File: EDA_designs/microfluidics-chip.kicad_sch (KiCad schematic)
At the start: 38 parts, among them J1 Conn_01x06_Pin, J10 39-53-2045, J11 Conn_01x14_Pin, J12 Conn_01x14_Pin, J13 39-53-2045, J14 39-53-2045, J15 Conn_ARM_SWD_TagConnect_TC2030, J16 Conn_01x02_Socket, J18 EJ508A, J2 Conn_01x06_Pin, J3 Conn_01x06_Pin, J4 Conn_01x06_Pin, J5 Conn_01x04_Socket, J8 39-53-2045, Q1 NDT3055L, Q3 NDT3055L, SW2 SW_Nidec_CAS-120A1, U1 LM2576HVS-3.3, U4 LM2576HVS-5, U6 STM32F410C8Tx

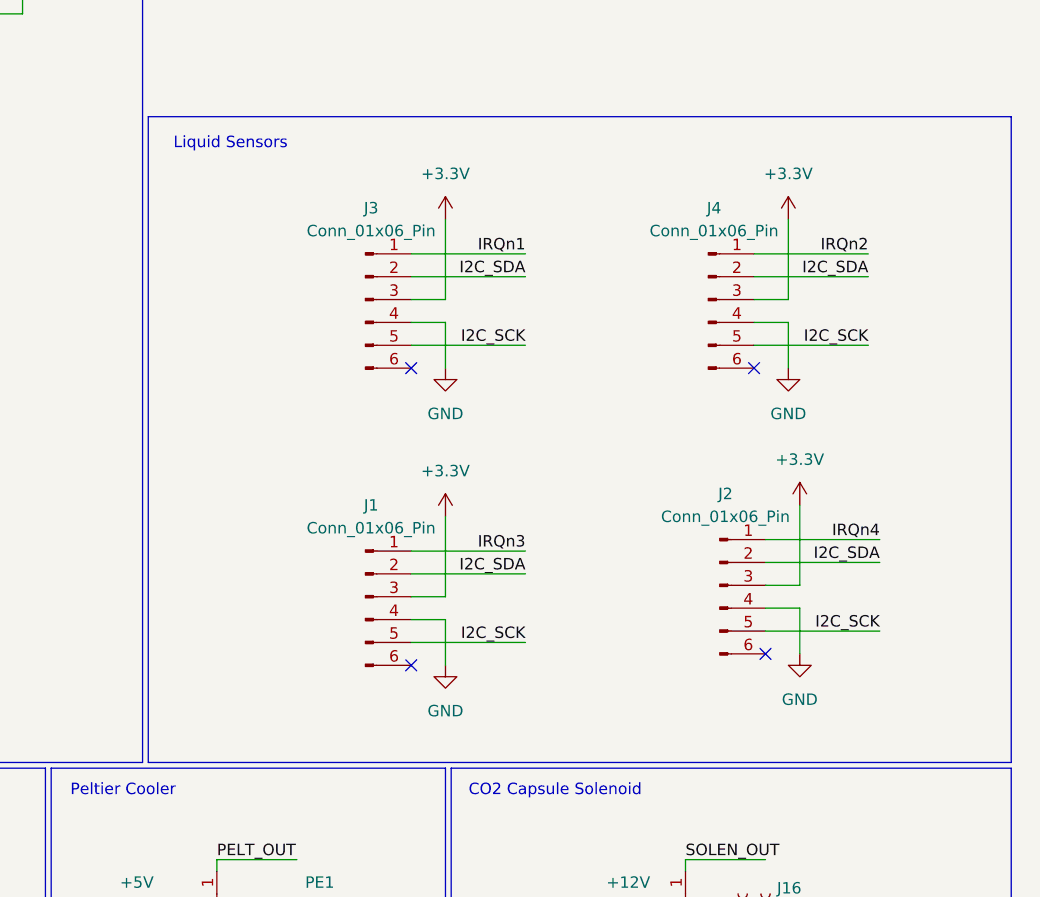
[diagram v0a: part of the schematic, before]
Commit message: Pushing v3
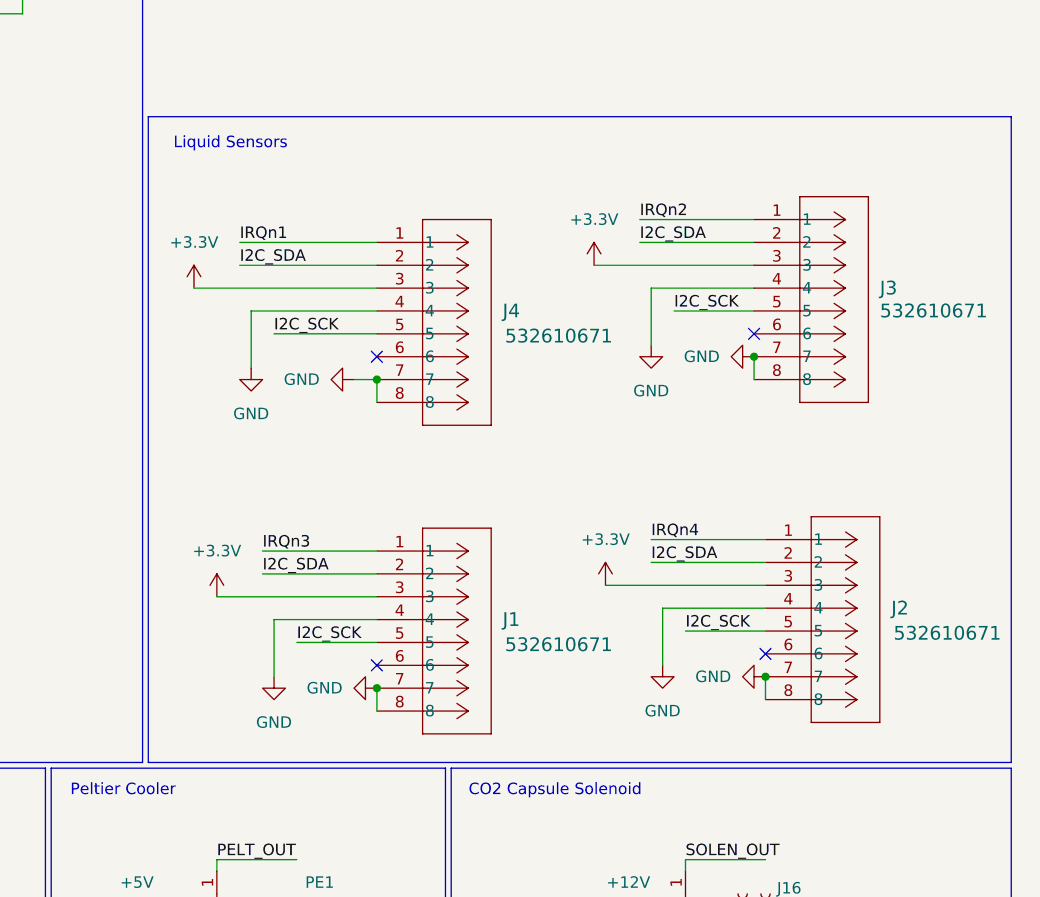
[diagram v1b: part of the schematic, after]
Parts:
- removed J1, J2, J3, J4: Conn_01x06_Pin, Connector_Hirose:Hirose_DF13-06P-1.25DSA_1x06_P1.25mm_Vertical, symbol Connector:Conn_01x06_Pin
- added J1, J2, J3, J4: 532610671, co2_sensor_footprint:CON_532610671, symbol co2_sensor_molex_footprint:532610671
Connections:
- net +3.3V: now also J1.3, J2.3, J3.3, J4.3
- net GND: now also J1.4, J1.7, J1.8, J2.4, J2.7, J2.8, J3.4, J3.7, J3.8, J4.4, J4.7, J4.8
- net I2C_SCK: now also J1.5, J2.5, J3.5, J4.5
- net I2C_SDA: now also J1.2, J2.2, J3.2, J4.2
- net IRQn1: now also J4.1
- net IRQn2: now also J3.1
- net IRQn3: now also J1.1
- net IRQn4: now also J2.1
